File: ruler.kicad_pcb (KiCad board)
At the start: 2 copper layers, 159.1 x 29.1 mm, 1 part, among them J1 Conn_01x01

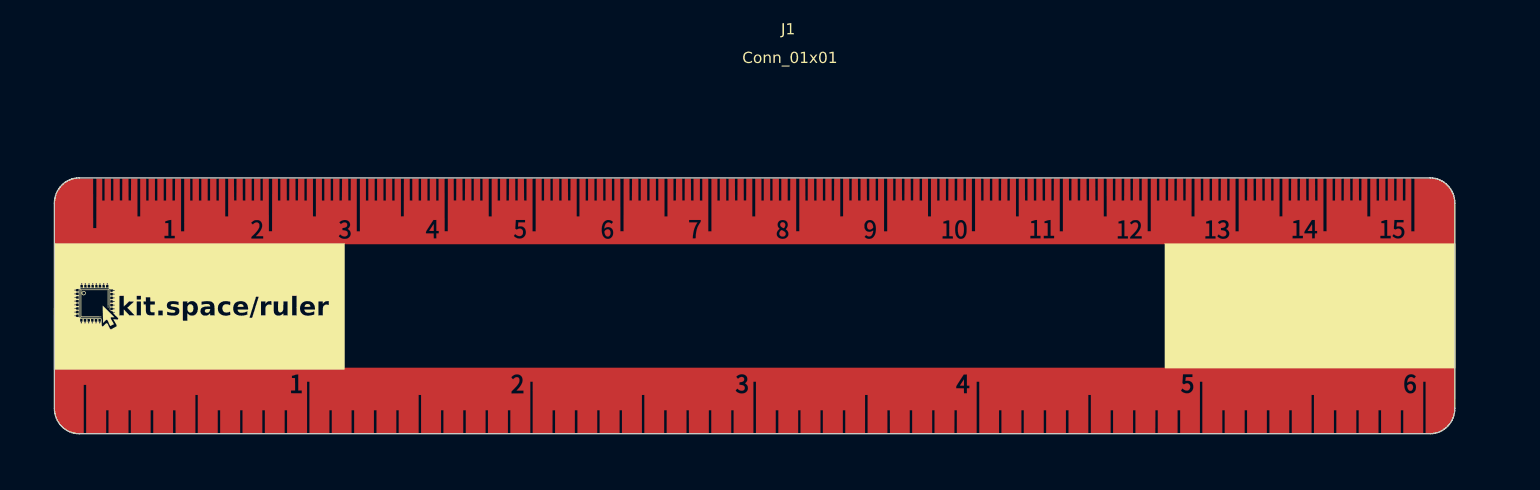
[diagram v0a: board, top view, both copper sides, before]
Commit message: Clear out old stuff, include drawing as module
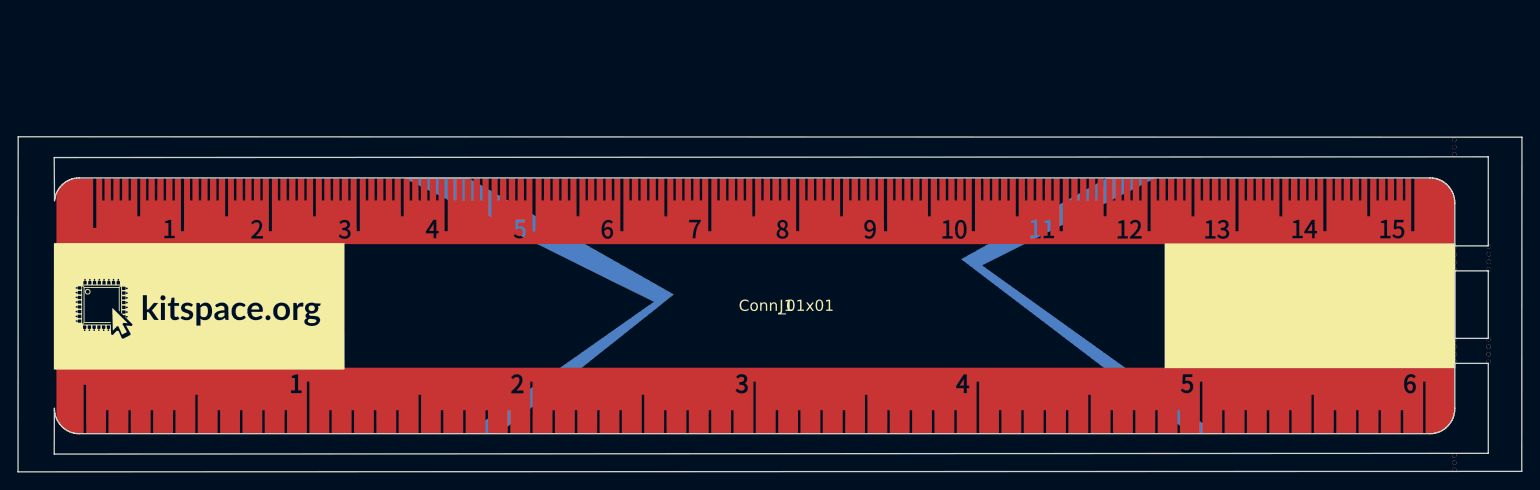
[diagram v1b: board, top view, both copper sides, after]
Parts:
- J1: footprint custom:pcbart -> drawing:drawing
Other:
- board size 159.1 x 29.1 mm -> 170.8 x 38.1 mm
